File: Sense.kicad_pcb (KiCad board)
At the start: 2 copper layers, 18.4 x 10.2 mm, 12 parts, among them J1 Callistated 1, J2 Callistated 2, U1 LSM6DS3TR-C, U2 LPS22HB, U3 LIS2MDL, U4 H3LIS100DLTR

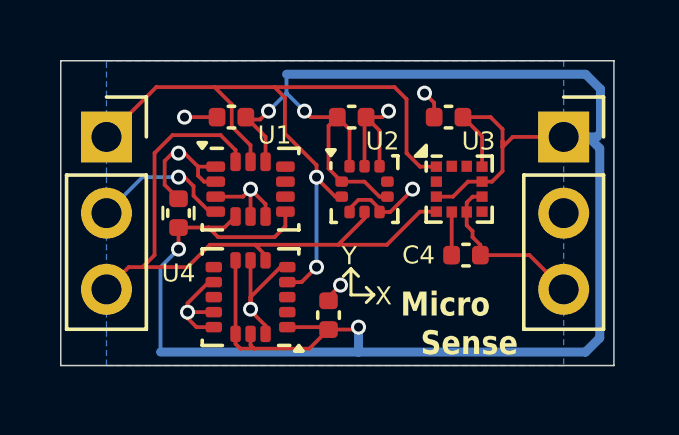
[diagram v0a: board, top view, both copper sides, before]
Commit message: Updated after review
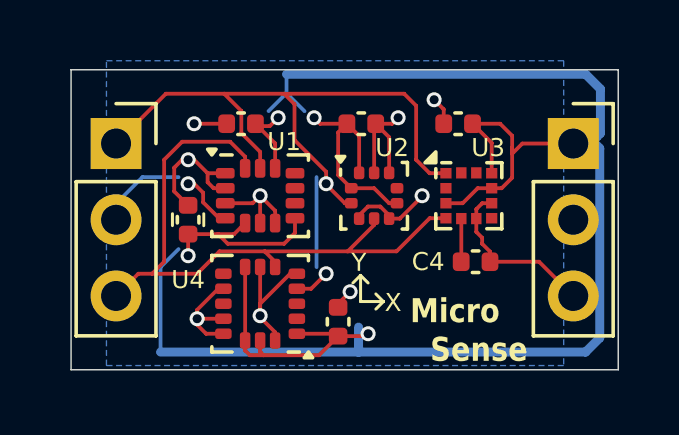
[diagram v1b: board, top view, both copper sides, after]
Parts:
- moved C2 0.39 mm to (142.1, 96.1)
- moved U2 0.39 mm to (142.5, 98.5)
- moved C1 0.39 mm to (138.1, 96.1)
- moved C3 0.39 mm to (145.3, 96.1)
- moved U4 0.39 mm to (138.7, 102.1)
- moved C4 0.39 mm to (145.9, 100.7)
- moved C5 0.39 mm to (136.3, 99.3)
- moved C6 0.39 mm to (141.3, 102.7)
- moved J1 0.39 mm to (133.9, 96.7)
- moved J2 0.39 mm to (149.2, 96.7)
- moved U1 0.39 mm to (138.7, 98.5)
- moved U3 0.39 mm to (145.7, 98.5)
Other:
- board size 18.4 x 10.2 mm -> 18.2 x 10 mm
